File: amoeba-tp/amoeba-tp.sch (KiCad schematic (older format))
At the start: 32 parts

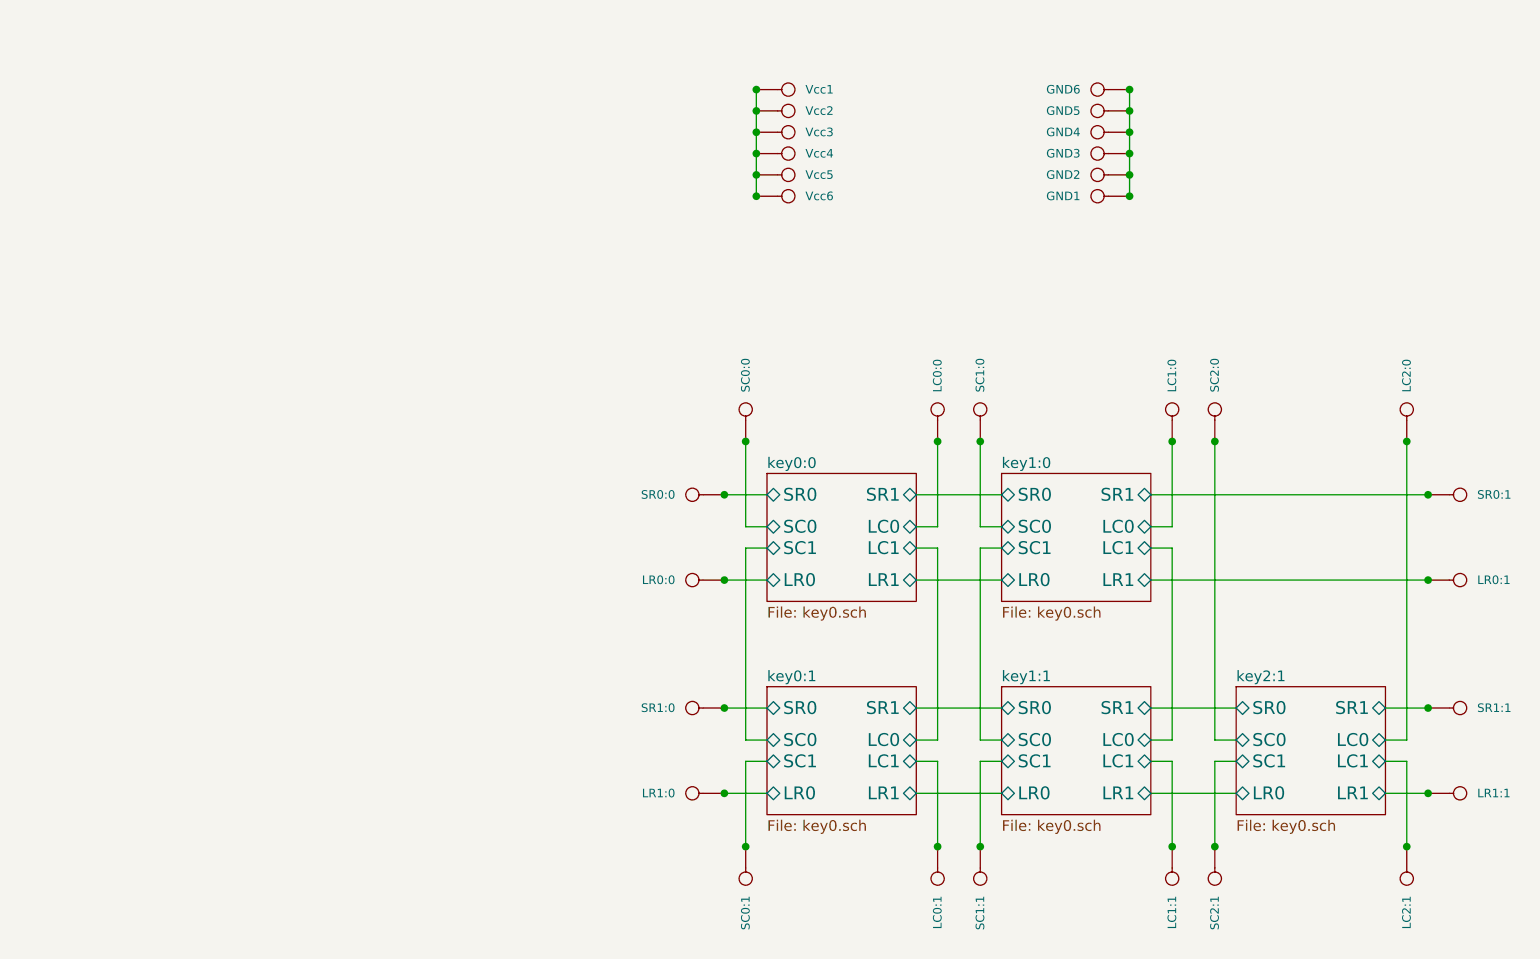
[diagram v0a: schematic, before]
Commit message: Cleaned up Amoeba TP design.
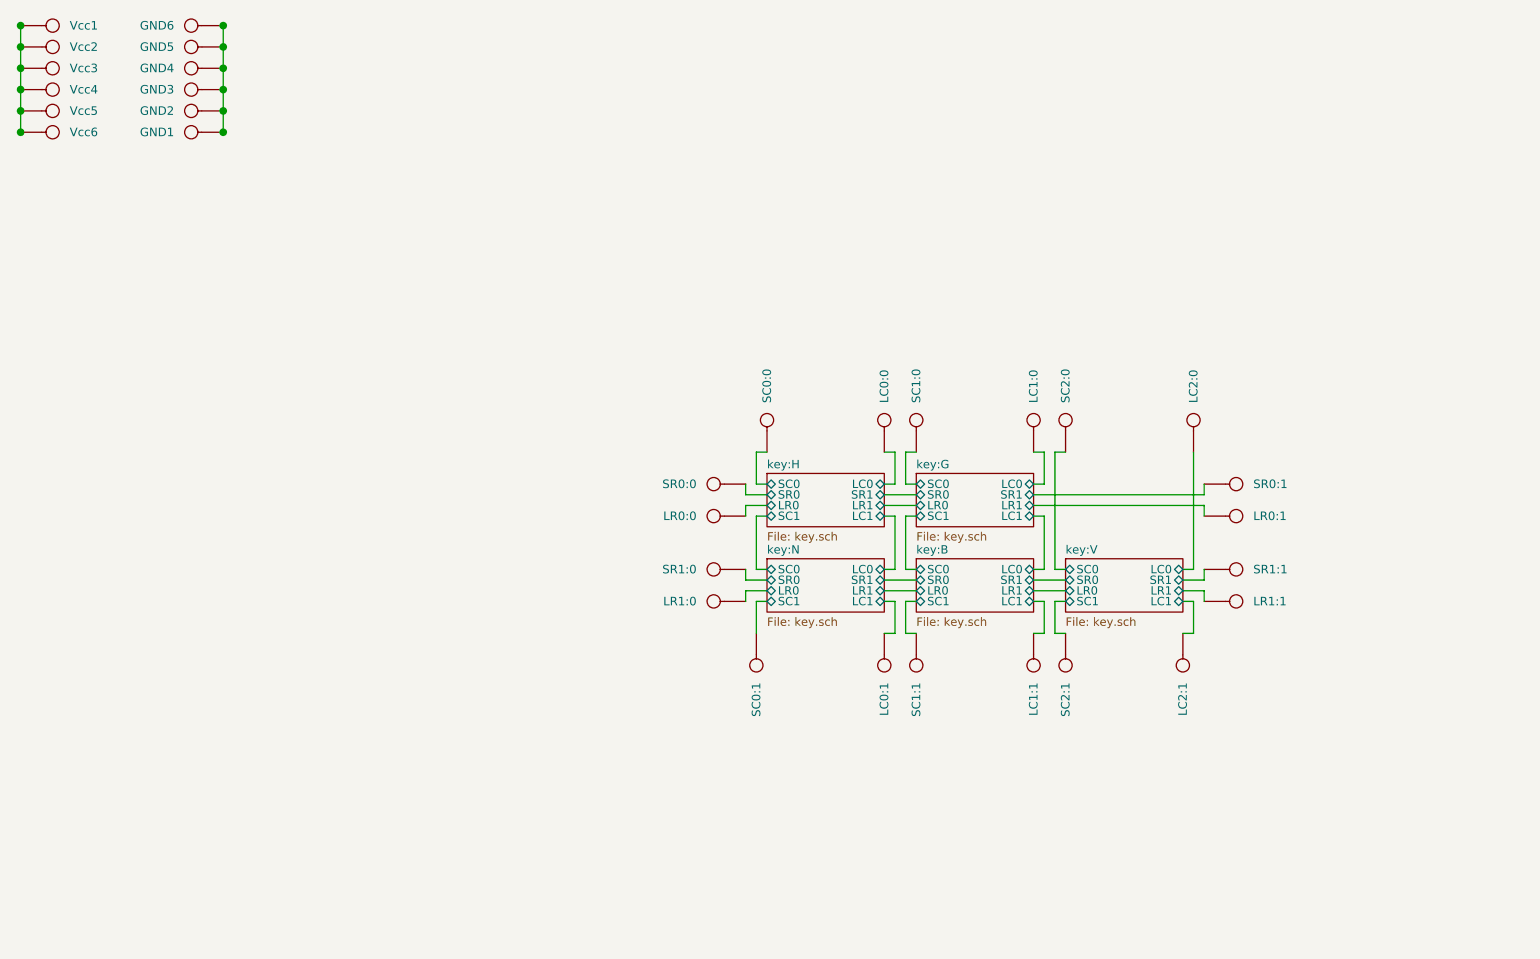
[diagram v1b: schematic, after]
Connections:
- net key0:0/LC0 renamed key:H/LC0
- net key0:0/LR0 renamed key:H/LR0
- net key0:0/SC0 renamed key:H/SC0
- net key0:0/SR0 renamed key:H/SR0
- net key0:1/LC1 renamed key:N/LC1
- net key0:1/LR0 renamed key:N/LR0
- net key0:1/SC1 renamed key:N/SC1
- net key0:1/SR0 renamed key:N/SR0
- net key1:0/LC0 renamed key:G/LC0
- net key1:0/LR1 renamed key:G/LR1
- net key1:0/SC0 renamed key:G/SC0
- net key1:0/SR1 renamed key:G/SR1
- net key1:1/LC1 renamed key:B/LC1
- net key1:1/SC1 renamed key:B/SC1
- net key2:1/LC0 renamed key:V/LC0
- net key2:1/LC1 renamed key:V/LC1
- net key2:1/LR1 renamed key:V/LR1
- net key2:1/SC0 renamed key:V/SC0
- net key2:1/SC1 renamed key:V/SC1
- net key2:1/SR1 renamed key:V/SR1
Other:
- moved on the sheet: GND1, GND2, GND3, GND4, GND5, GND6, LC0:0, LC0:1, LC1:0, LC1:1, LC2:0, LC2:1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
